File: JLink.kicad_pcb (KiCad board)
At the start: 2 copper layers, 76 parts

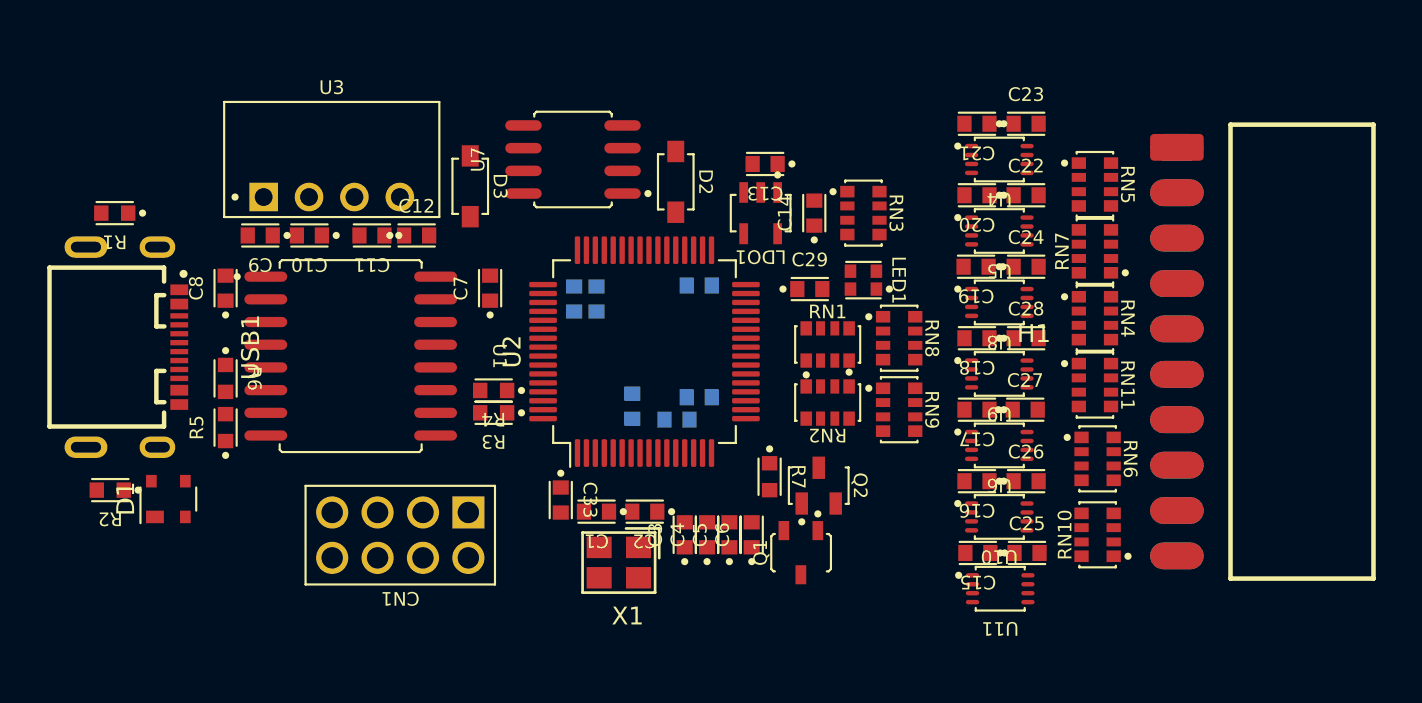
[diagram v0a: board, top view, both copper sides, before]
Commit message: 修改内容中
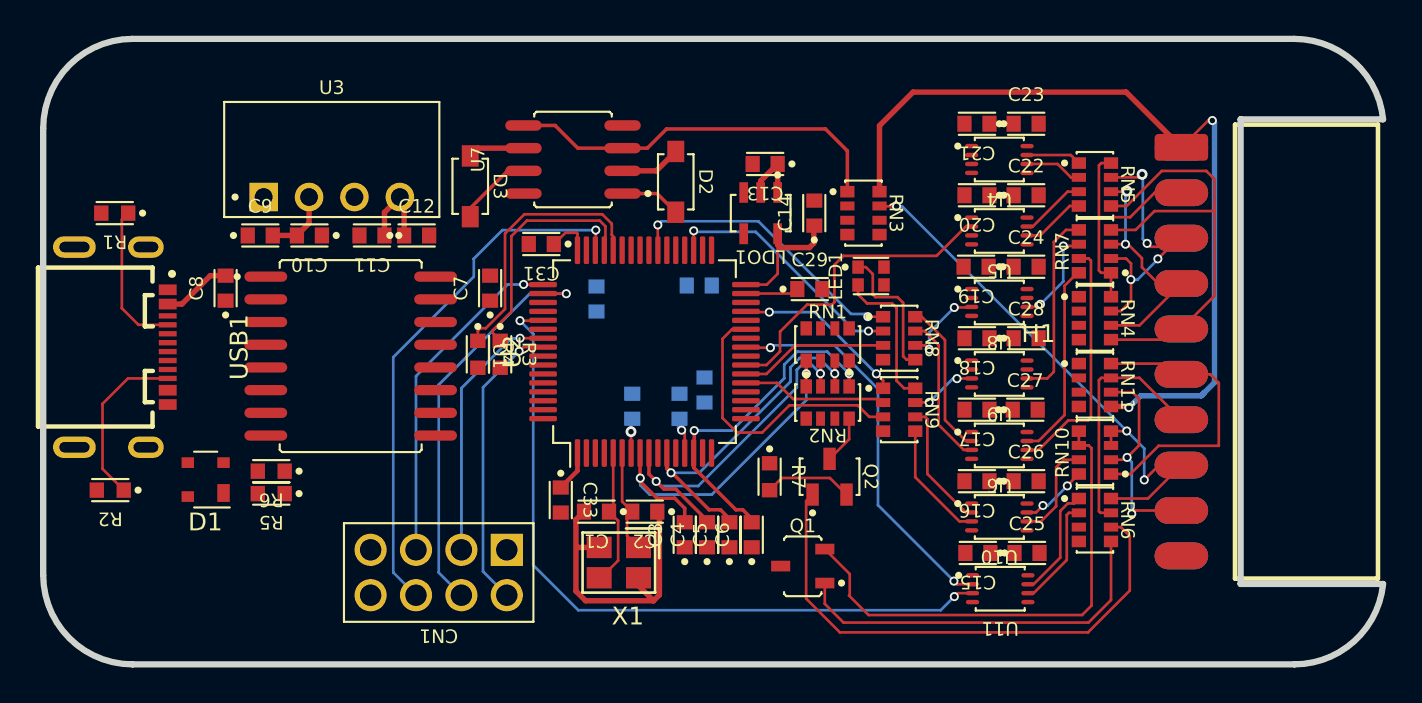
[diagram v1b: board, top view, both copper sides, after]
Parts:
- C31: moved to F.Cu
- moved R6 5.78 mm to (47.3, 82.2), turned to 180 degrees
- moved RN10 4.60 mm to (93.3, 81.2)
- moved R5 4.49 mm to (47.3, 83.4), turned to 180 degrees
- moved C31 3.58 mm to (62.4, 69.5), turned to 180 degrees
- moved RN6 3.42 mm to (93.3, 84.9)
- moved R3 3.30 mm to (60.1, 75.7), turned to -90 degrees
- moved CN1 3.00 mm to (56.6, 87.9)
- moved D1 2.35 mm to (43.6, 82.7), turned to 180 degrees
- moved R4 2.21 mm to (58.8, 75.7), turned to -90 degrees
- moved Q2 0.78 mm to (78.5, 82.5)
- moved C35 0.76 mm to (70.1, 78.6), turned to 90 degrees
- moved Q1 0.76 mm to (77.0, 87.5), turned to 0 degrees
- moved USB1 0.65 mm to (38.9, 75.2)
- moved C36 0.50 mm to (71.5, 77.7), turned to 90 degrees
- moved LED1 0.48 mm to (80.8, 71.3), turned to 90 degrees
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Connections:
- net /PDDM renamed /PDDN
- net Net-(U1-DD+) renamed /USB/DD+
- net Net-(U1-DD-) renamed /USB/DD-
- net Net-(U1-UD+) renamed /USB/UD+
- net Net-(U1-UD–) renamed /USB/UD-
- C7 pad 2: /USB/P5V -> P5V
- CN1 pad 6: /STM32/JTMS_SWDIO -> JTCK_SWDIO
- RN10 pad 5: Net-(U10-B1) -> Net-(Q1-Pad2)
- RN10 pad 6: Net-(U10-B2) -> Net-(Q1-Pad2)
- RN10 pad 7: Net-(Q1-Pad2) -> Net-(U10-B2)
- RN10 pad 8: Net-(Q1-Pad2) -> Net-(U10-B1)
- RN3 pad 5: TVRF -> Net-(Q2-B)
- RN3 pad 6: ENSRST -> 3V3
- RN3 pad 7: 3V3 -> ENSRST
- RN3 pad 8: Net-(Q2-B) -> TVRF
- U1 pad 16: /USB/P5V -> P5V
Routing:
- net TVRF: track 0.00 -> 49.9 mm, vias 0 -> 2
- net NDAT11: track 0.00 -> 41.3 mm, vias 0 -> 2
- net ENSRST: track 0.00 -> 31.0 mm, vias 0 -> 3
- net Net-(Q2-B): track 0.00 -> 30.1 mm
- net JTCK_SWDIO: track 0.00 -> 29.8 mm, vias 0 -> 1
- net Net-(Q1-Pad2): track 0.00 -> 27.8 mm
- net ETCK: track 0.00 -> 26.8 mm
- net JTDI: track 0.00 -> 22.9 mm, vias 0 -> 1
- net NDAT12: track 0.00 -> 22.1 mm, vias 0 -> 2
- net Net-(U7-+INA): track 0.00 -> 21.9 mm
- net Net-(Q1-Pad1): track 0.00 -> 21.4 mm
- net /ADC3: track 0.00 -> 21.0 mm, vias 0 -> 2
- net /ADC1: track 0.00 -> 20.5 mm, vias 0 -> 2
- net /ADC2: track 0.00 -> 20.0 mm, vias 0 -> 2
- net /ADC4: track 0.00 -> 19.6 mm, vias 0 -> 2
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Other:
- board outline added: 75 x 35 mm
- copper layers 2 -> 4
